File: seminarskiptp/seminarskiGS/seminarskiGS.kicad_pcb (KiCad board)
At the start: 2 copper layers, 13 parts, among them J1 Screw_Terminal_01x02, SW1 SW_Push, U1 AT89C4051-24P, U2 LCD-016N002L, U3 HC-SR04, Y1 11.0592MHz

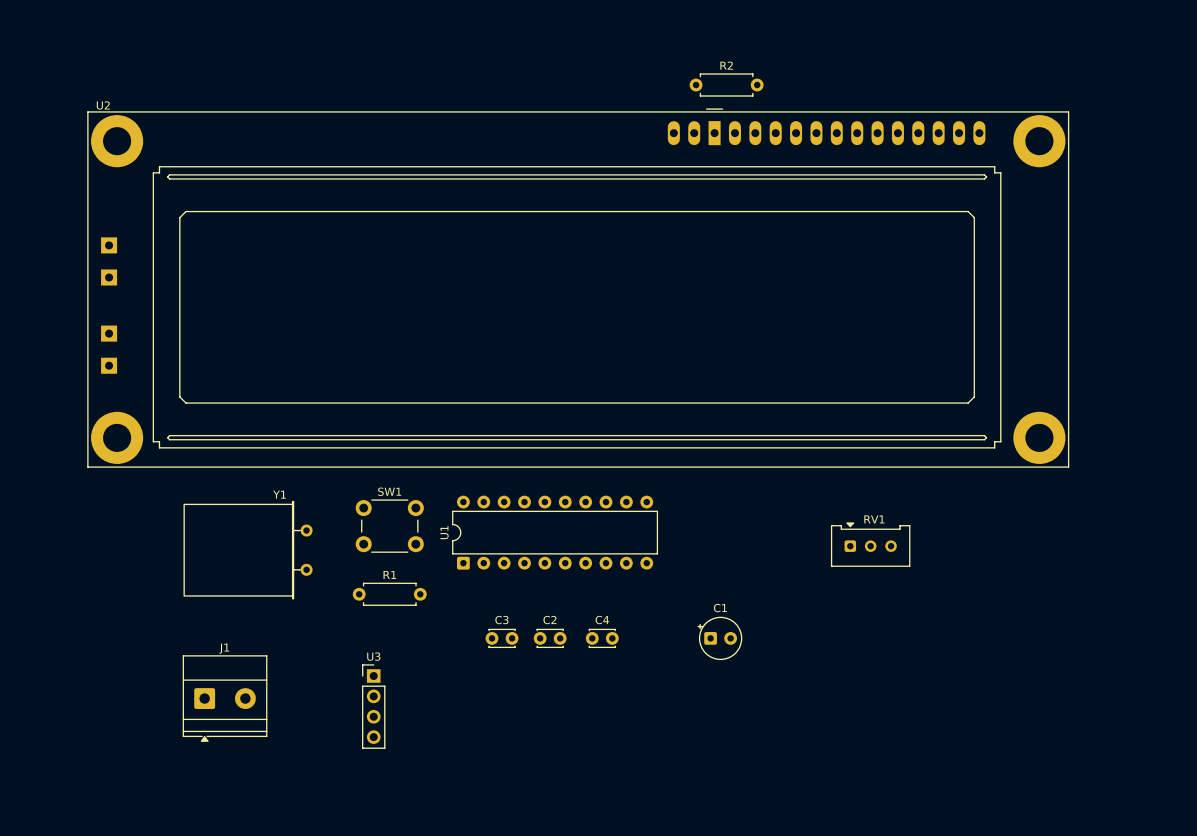
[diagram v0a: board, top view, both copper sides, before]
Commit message: 27.11
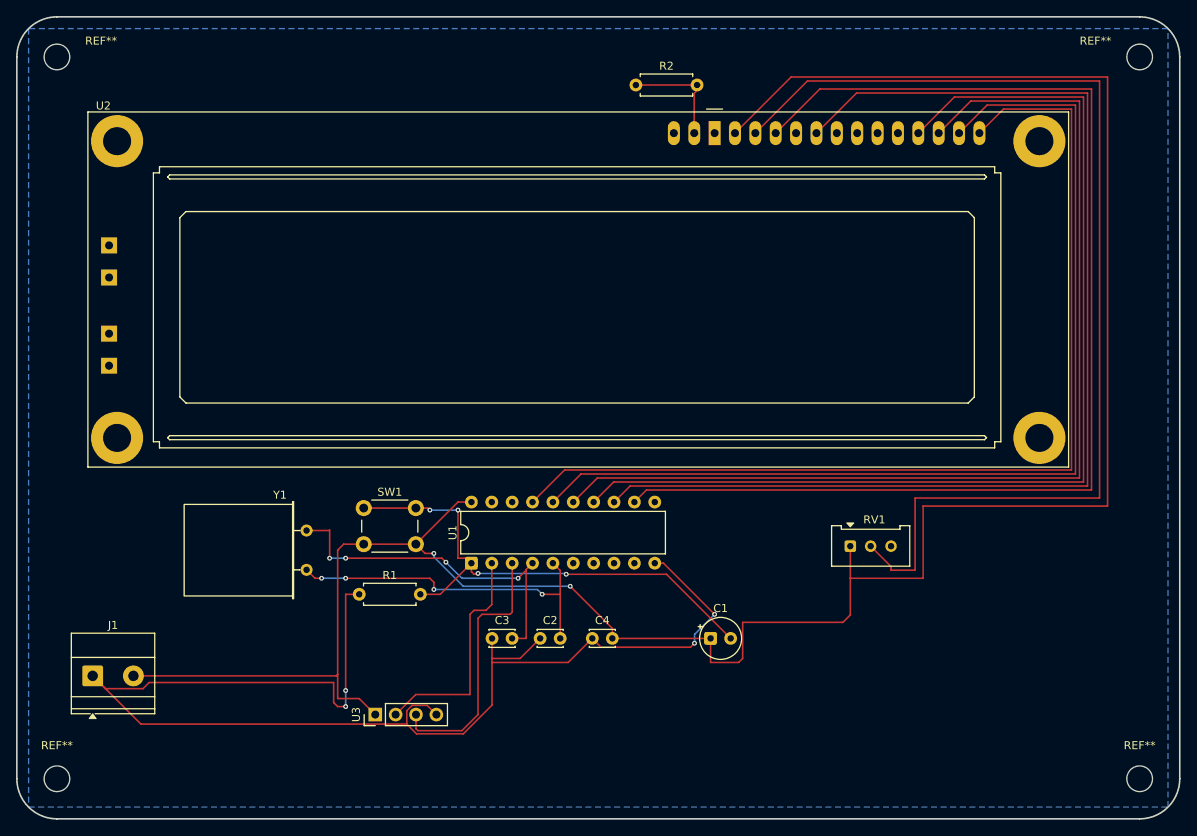
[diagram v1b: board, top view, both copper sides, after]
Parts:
- added REF**: MountingHole_3.2mm_M3, MountingHole:MountingHole_3.2mm_M3, F.Cu at (220.0, 35.0)
- added REF**: MountingHole_3.2mm_M3, MountingHole:MountingHole_3.2mm_M3, F.Cu at (220.0, 125.0)
- added REF**: MountingHole_3.2mm_M3, MountingHole:MountingHole_3.2mm_M3, F.Cu at (85.0, 125.0)
- added REF**: MountingHole_3.2mm_M3, MountingHole:MountingHole_3.2mm_M3, F.Cu at (85.0, 35.0)
- moved J1 14.2 mm to (89.5, 112.2)
- moved R2 7.50 mm to (157.2, 38.5)
- moved U3 4.81 mm to (124.7, 117.0), turned to 90 degrees
- moved U1 1.00 mm to (136.7, 98.1)
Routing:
- net +5V: track 0.00 -> 289.4 mm, vias 0 -> 2
- net GND: track 0.00 -> 168.6 mm, vias 0 -> 4
- net Net-(U1-P1.0): track 0.00 -> 149.3 mm
- net Net-(U1-P1.1): track 0.00 -> 144.7 mm
- net Net-(U2-VO): track 0.00 -> 136.7 mm
- net Net-(U1-P1.2): track 0.00 -> 132.6 mm
- net Net-(U1-P1.3): track 0.00 -> 130.6 mm
- net Net-(U1-P1.4): track 0.00 -> 128.6 mm
- net Net-(U1-P1.5): track 0.00 -> 126.6 mm
- net Net-(U1-RST/VPP): track 0.00 -> 64.7 mm, vias 0 -> 4
- net Net-(U1-XTAL2): track 0.00 -> 43.8 mm, vias 0 -> 4
- net Net-(U1-XTAL1): track 0.00 -> 43.2 mm, vias 0 -> 4
- net Net-(U1-P3.1): track 0.00 -> 33.1 mm
- net Net-(U1-P3.0): track 0.00 -> 28.7 mm
- net +5C: track 0.00 -> 14.1 mm
- added copper zone on B.Cu, net GND
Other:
- board outline added: 145 x 100 mm
